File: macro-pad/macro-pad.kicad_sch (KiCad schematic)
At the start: 4 parts, among them SW1 SW_Push, SW2 SW_Push, SW3 SW_Push, U1 MOUDLE-SEEEDUINO-XIAO

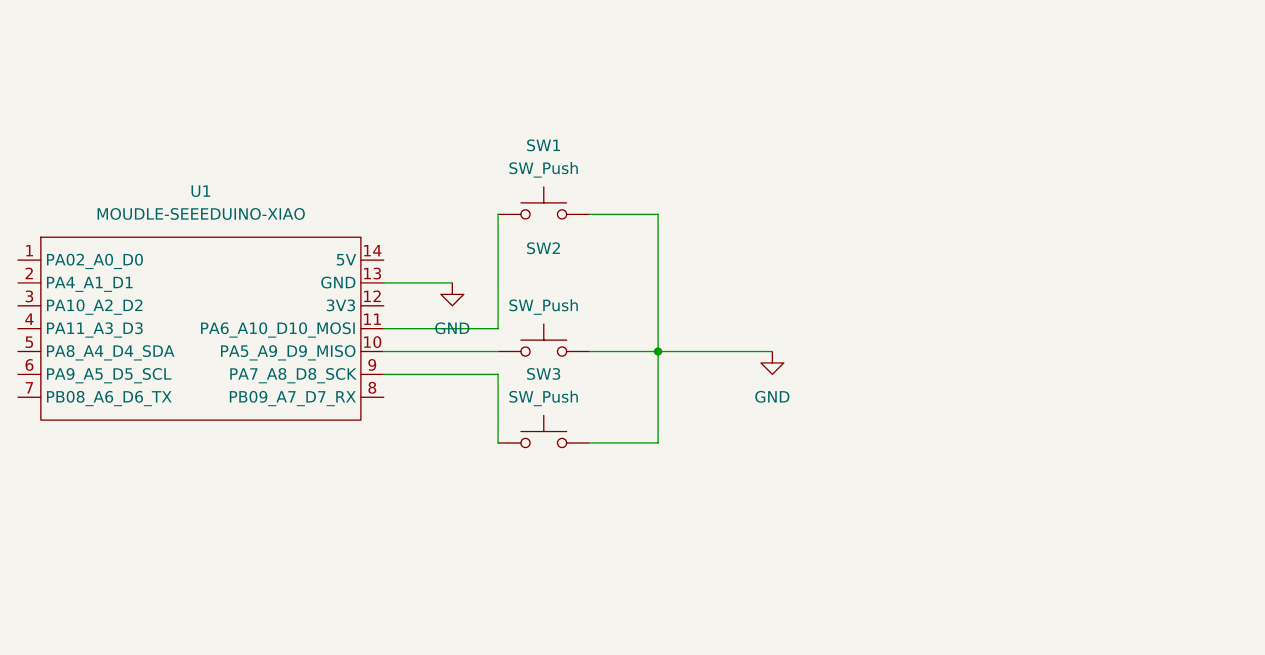
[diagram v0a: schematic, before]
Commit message: added gerber files
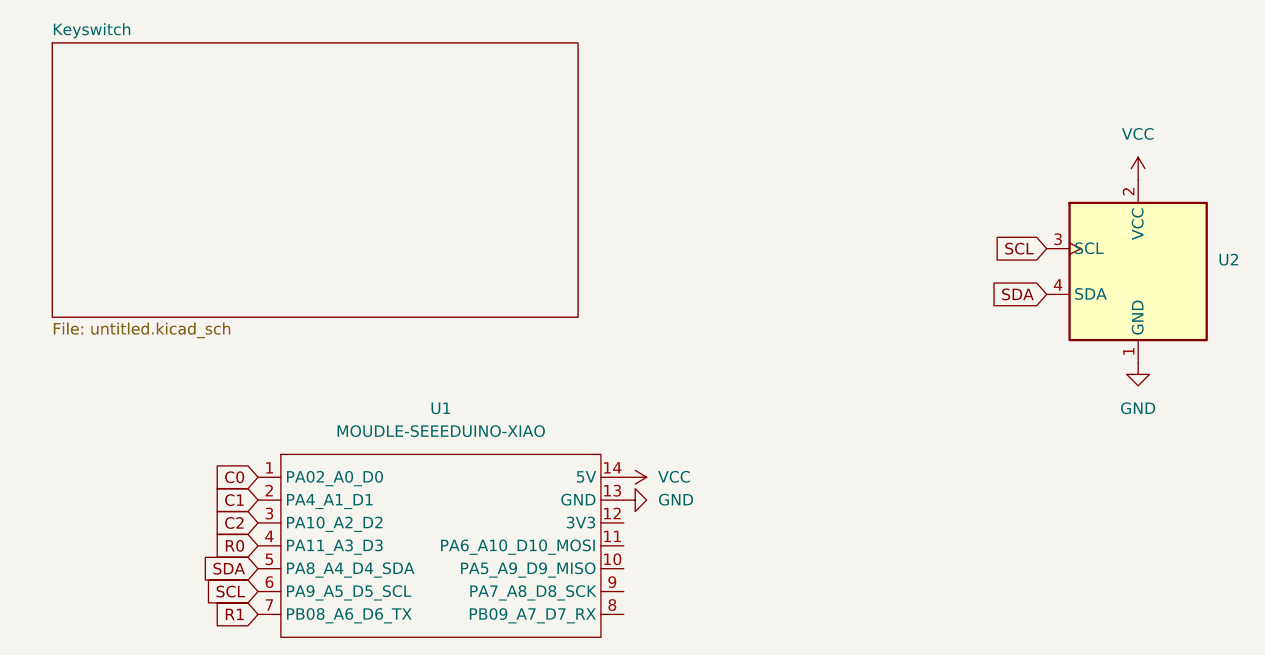
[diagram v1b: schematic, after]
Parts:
- removed SW1, SW2, SW3: SW_Push, Button_Switch_Keyboard:SW_Cherry_MX_1.00u_PCB, symbol Switch:SW_Push
- added U2: ER_OLEDM0.91_1x-I2C, KiCad-SSD1306-0.91-OLED-4pin-128x32:SSD1306-0.91-OLED-4pin-128x32, symbol Display_Graphic:ER_OLEDM0.91_1x-I2C
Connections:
- net GND: now also U2.1 (GND)
- net C0: now reaches U1.1 (PA02_A0_D0)
- net VCC: now reaches U1.14 (5V)
- net VCC: now also U2.2 (VCC)
- net C1: now reaches U1.2 (PA4_A1_D1)
- net C2: now reaches U1.3 (PA10_A2_D2)
- net R0: now reaches U1.4 (PA11_A3_D3)
- net SDA: now reaches U1.5 (PA8_A4_D4_SDA)
- net SDA: now also U2.4 (SDA)
- net SCL: now reaches U1.6 (PA9_A5_D5_SCL)
- net SCL: now also U2.3 (SCL)
- net R1: now reaches U1.7 (PB08_A6_D6_TX)
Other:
- added sheet Keyswitch (untitled.kicad_sch)
